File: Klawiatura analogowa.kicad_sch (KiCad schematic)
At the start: 33 parts, among them J1 USB_C_Receptacle_USB2.0, J2 Conn_01x04_Pin, U1 SN74LV1T34DBV, U18 STM32F072CBT6, U19 CD74HC4067SM, U2 XC6206P332MR-Regulator_Linear, U20 PRTR5V0U2X

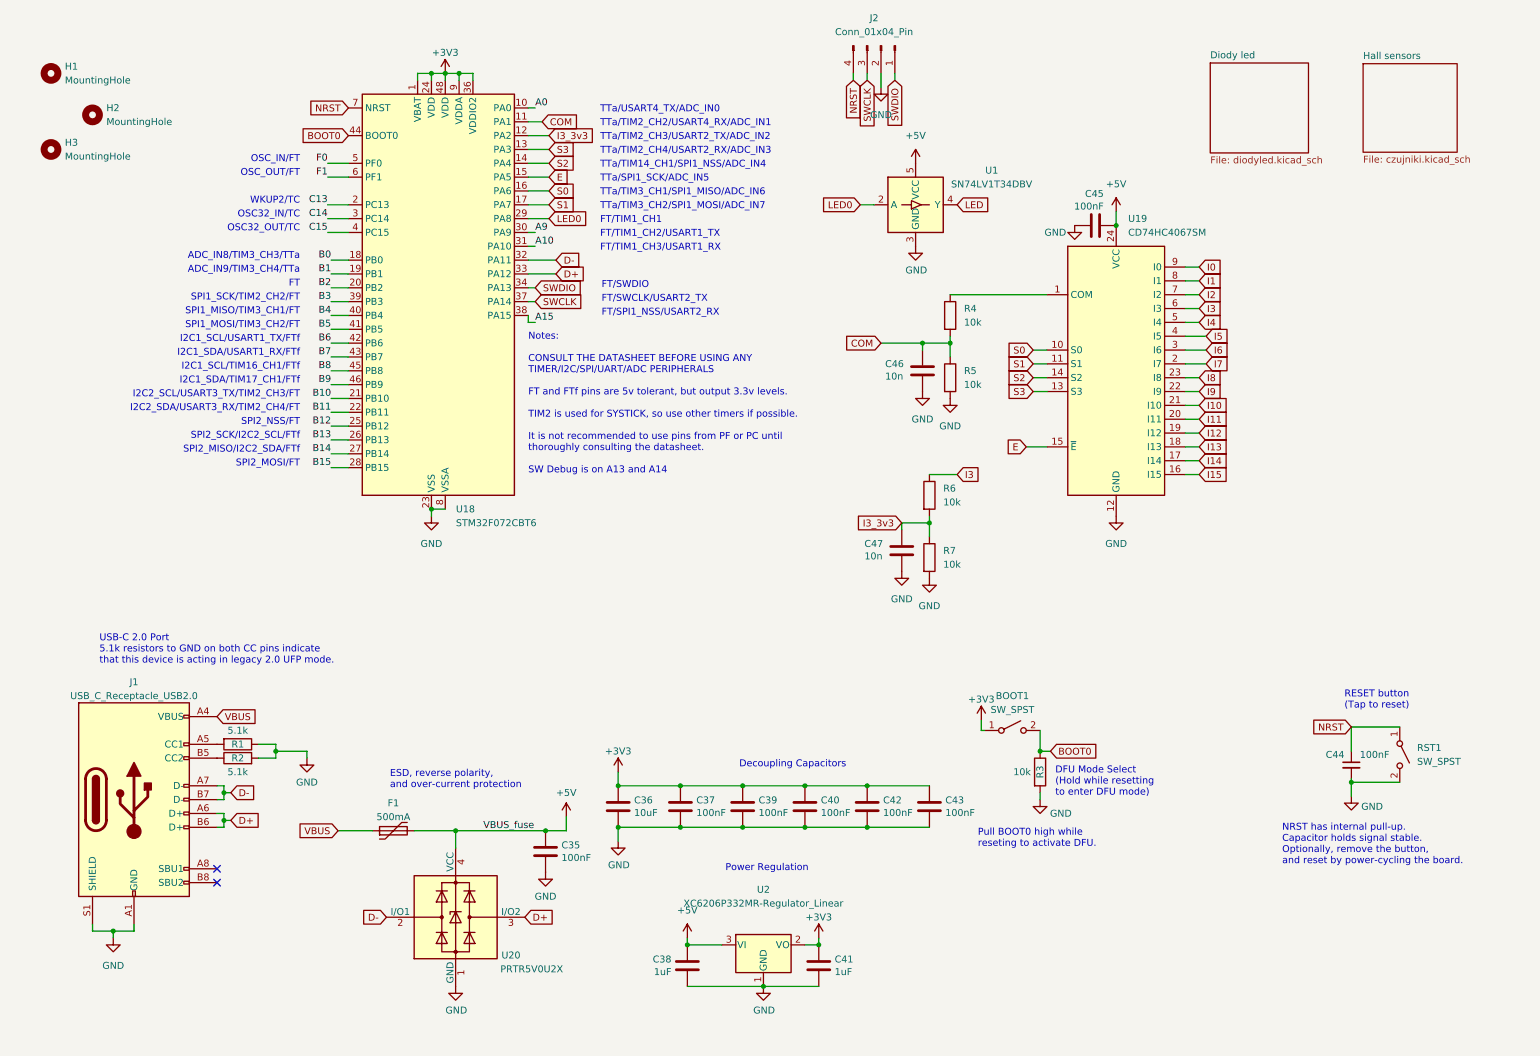
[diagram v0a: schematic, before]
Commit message: Poprawiono wygląd schematu
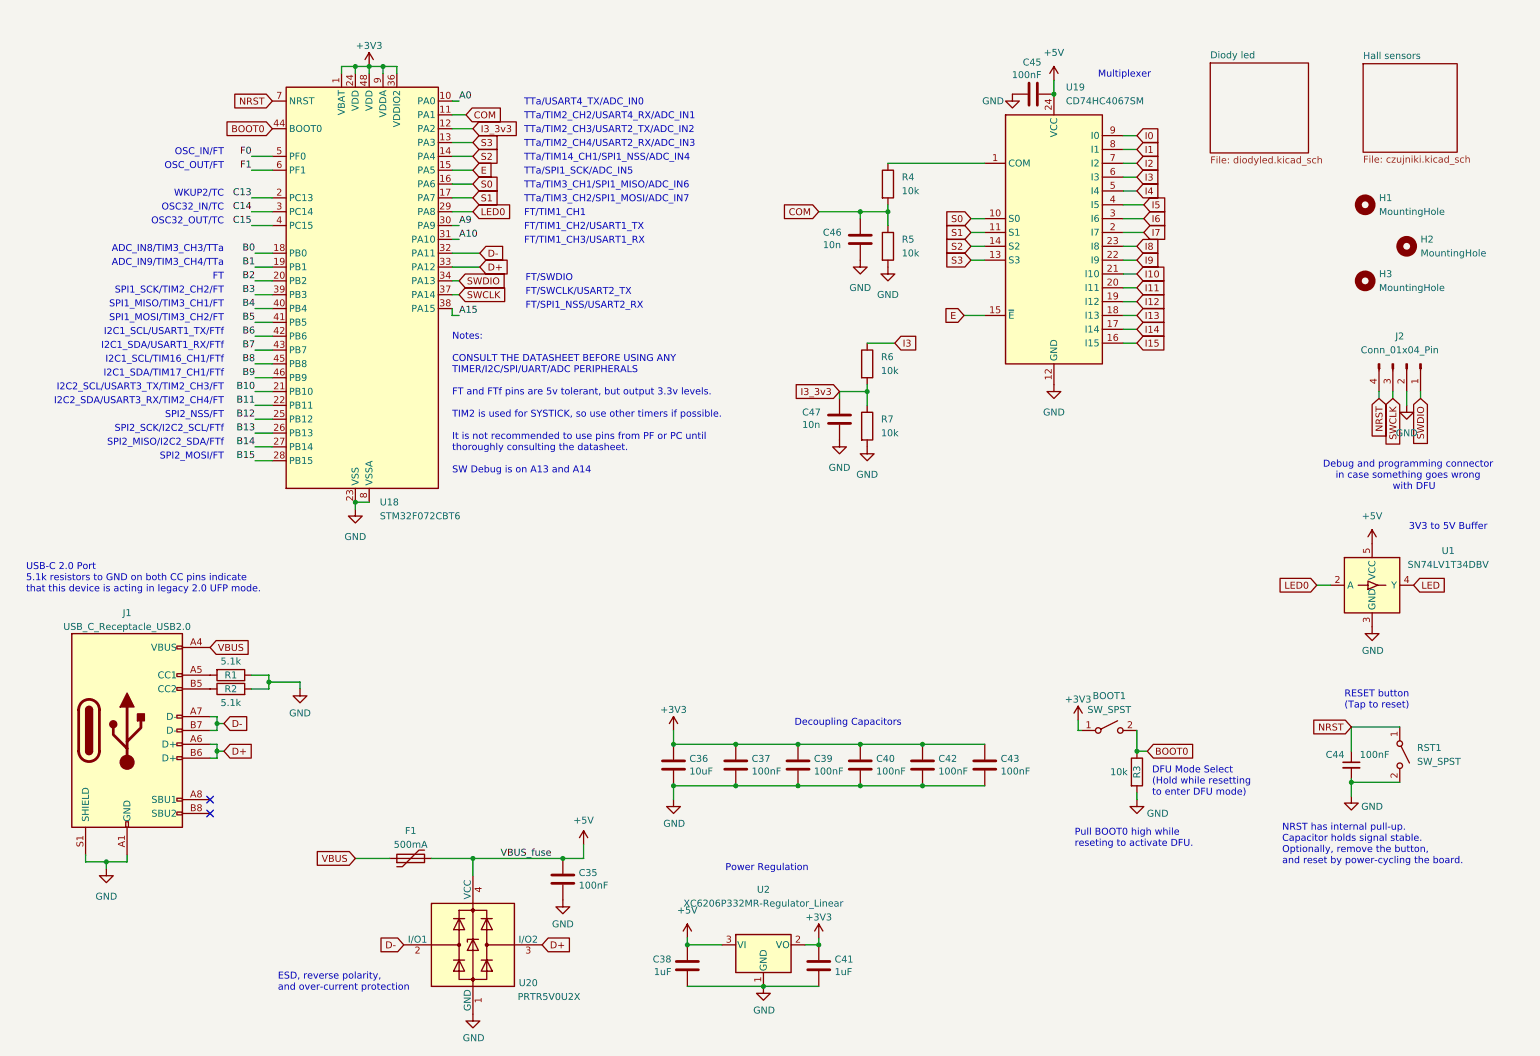
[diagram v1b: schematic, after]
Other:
- note added: "3V3 to 5V Buffer"
- note added: "Debug and programming connector in case something goes wrong with DFU"
- note added: "Multiplexer"
- moved on the sheet: BOOT1, C35, C36, C37, C39, C40, C42, C43, C45, C46, C47, F1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
